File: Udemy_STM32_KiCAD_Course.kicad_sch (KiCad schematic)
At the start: 24 parts, among them J1 USB_B_Micro, J2 Conn_01x04_Pin, SW1 SW_SPDT, U1 STM32F103C8T6, U2 AMS1117-3.3, Y1 16MHz

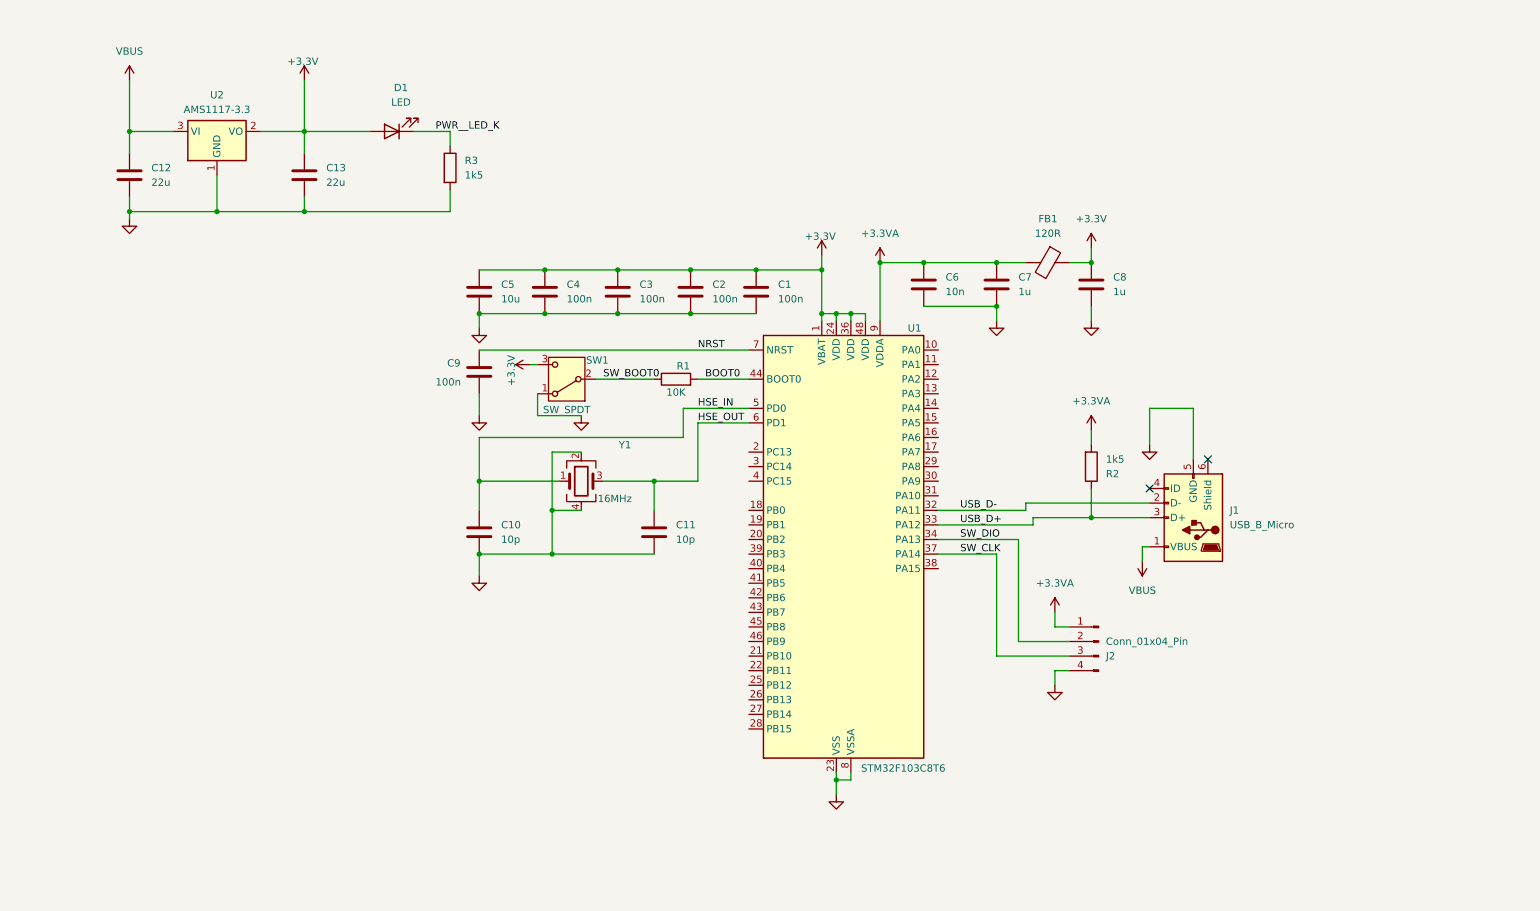
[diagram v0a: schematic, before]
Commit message: complete schematic and annotations
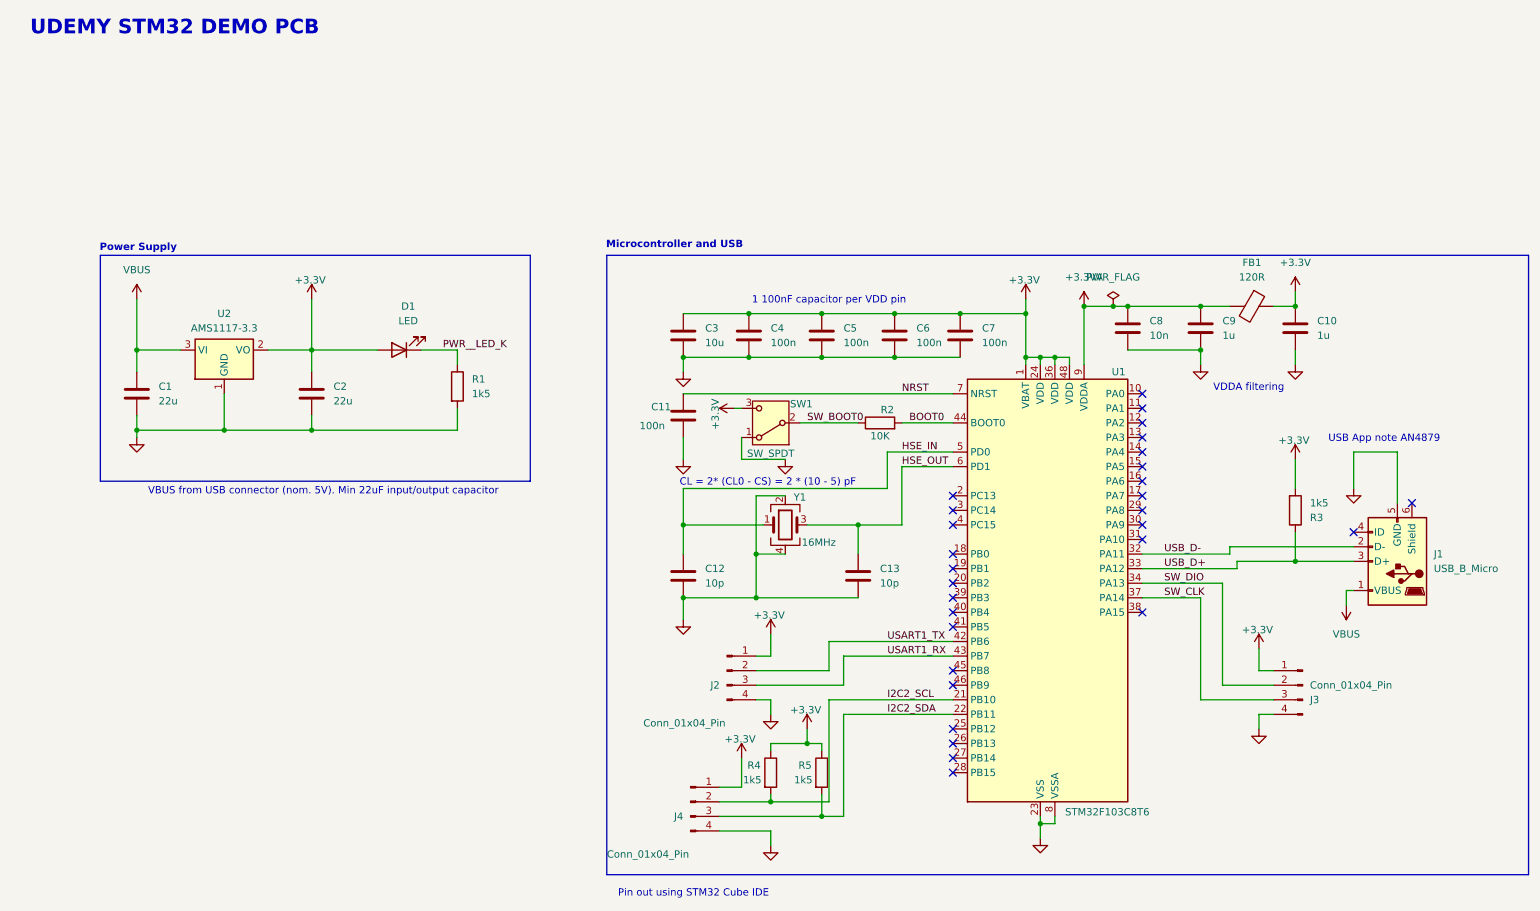
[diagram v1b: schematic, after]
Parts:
- added J2, J4: Conn_01x04_Pin, Connector_PinHeader_2.54mm:PinHeader_1x04_P2.54mm_Vertical, symbol Connector:Conn_01x04_Pin
- added R4, R5: 1k5, Resistor_SMD:R_0402_1005Metric, symbol Device:R
- C1: renamed from C12; footprint (none) -> Capacitor_SMD:C_0805_2012Metric
- C10: renamed from C8; footprint (none) -> Capacitor_SMD:C_0402_1005Metric
- C11: renamed from C9; footprint (none) -> Capacitor_SMD:C_0402_1005Metric
- C12: renamed from C10; footprint (none) -> Capacitor_SMD:C_0402_1005Metric
- C13: renamed from C11; footprint (none) -> Capacitor_SMD:C_0402_1005Metric
- C2: renamed from C13; footprint (none) -> Capacitor_SMD:C_0805_2012Metric
- C3: renamed from C5; footprint (none) -> Capacitor_SMD:C_0603_1608Metric
- C4: footprint (none) -> Capacitor_SMD:C_0402_1005Metric
- C5: renamed from C3; footprint (none) -> Capacitor_SMD:C_0402_1005Metric
- C6: renamed from C2; footprint (none) -> Capacitor_SMD:C_0402_1005Metric
- C7: renamed from C1; footprint (none) -> Capacitor_SMD:C_0402_1005Metric
- C8: renamed from C6; footprint (none) -> Capacitor_SMD:C_0402_1005Metric
- C9: renamed from C7; footprint (none) -> Capacitor_SMD:C_0402_1005Metric
- D1: footprint (none) -> LED_SMD:LED_0603_1608Metric
- FB1: footprint (none) -> Inductor_SMD:L_0603_1608Metric
- J1: footprint (none) -> Connector_USB:USB_Micro-B_Wuerth_629105150521
- J3: renamed from J2; footprint (none) -> Connector_PinHeader_2.54mm:PinHeader_1x04_P2.54mm_Vertical
- R1: renamed from R3; footprint (none) -> Resistor_SMD:R_0402_1005Metric
- R2: renamed from R1; footprint (none) -> Resistor_SMD:R_0402_1005Metric
- R3: renamed from R2; footprint (none) -> Resistor_SMD:R_0402_1005Metric
- SW1: footprint (none) -> Button_Switch_THT:SW_E-Switch_EG1224_SPDT_Angled
- Y1: footprint (none) -> Crystal:Crystal_SMD_3225-4Pin_3.2x2.5mm
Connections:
- net +3.3V: now also J3.1 (Pin_1), R3.2, J2.1 (Pin_1), J4.1 (Pin_1), R4.1, R5.1
- net +3.3VA: no longer J3.1 (Pin_1), R3.2
- net GND: now also J2.4 (Pin_4), J4.4 (Pin_4)
- net I2C2_SCL: now reaches U1.21 (PB10)
- net I2C2_SCL: now also J4.2 (Pin_2), R4.2
- net I2C2_SDA: now reaches U1.22 (PB11)
- net I2C2_SDA: now also J4.3 (Pin_3), R5.2
- net USART1_TX: now reaches U1.42 (PB6)
- net USART1_TX: now also J2.2 (Pin_2)
- net USART1_RX: now reaches U1.43 (PB7)
- net USART1_RX: now also J2.3 (Pin_3)
- no-connect marks 2 -> 29
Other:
- note added: "1 100nF capacitor per VDD pin"
- note added: "CL = 2* (CL0 - CS) = 2 * (10 - 5) pF"
- note added: "Microcontroller and USB"
- note added: "Pin out using STM32 Cube IDE"
- note added: "Power Supply"
- note added: "UDEMY STM32 DEMO PCB"
- note added: "USB App note AN4879"
- note added: "VBUS from USB connector (nom. 5V). Min 22uF input/output capacitor"
- note added: "VDDA filtering"
- title: (none) -> Udemy STM32 Demo PCB
- moved on the sheet: C1, C10, C11, C12, C13, C2, C3, C4, C5, C6, C7, C8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
